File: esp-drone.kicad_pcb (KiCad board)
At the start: 4 copper layers, 72.8 x 72.8 mm, 0 parts

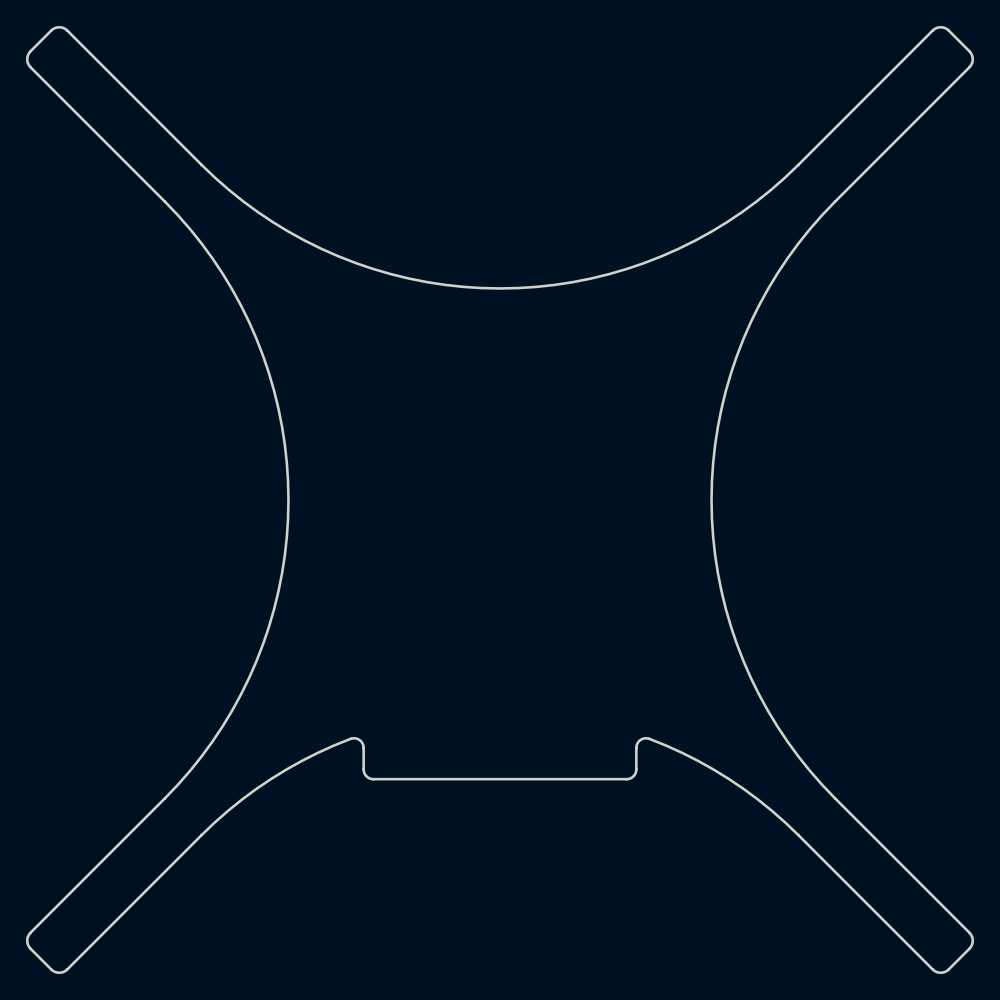
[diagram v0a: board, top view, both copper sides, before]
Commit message: .
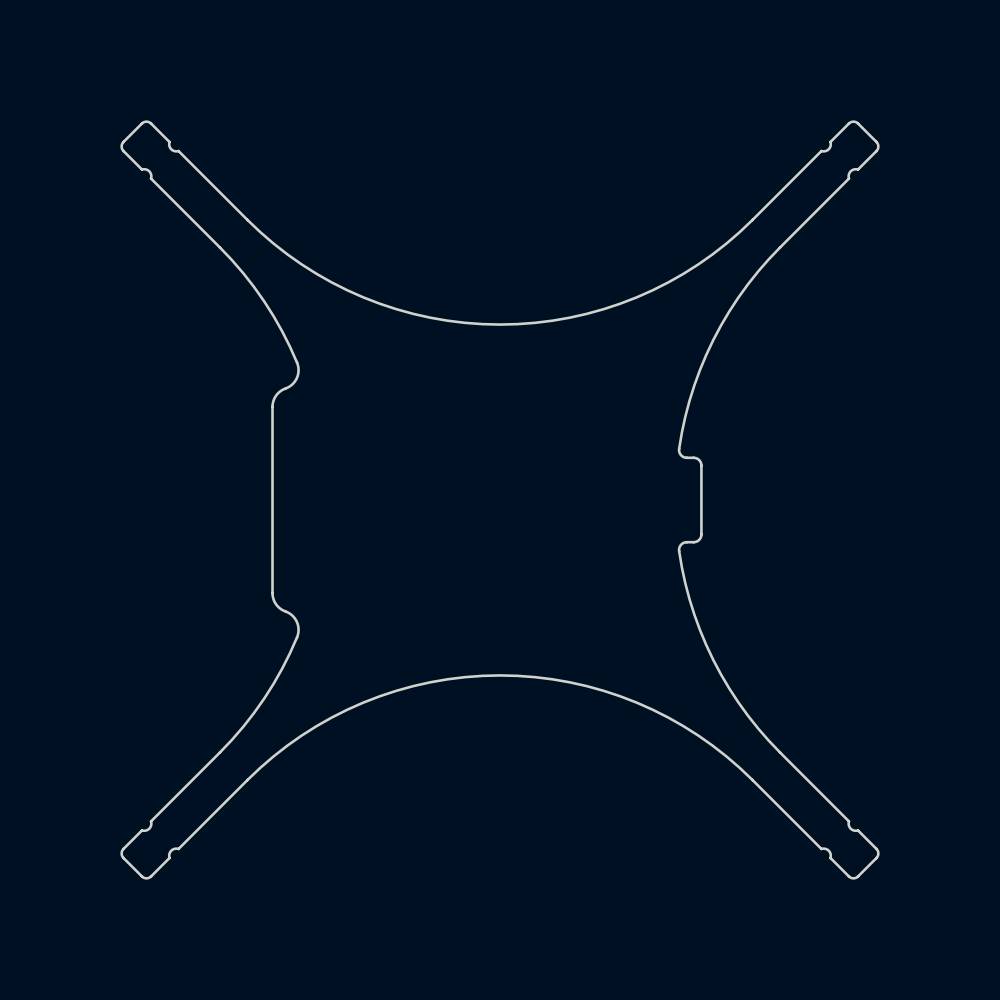
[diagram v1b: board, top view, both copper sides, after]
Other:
- board size 72.8 x 72.8 mm -> 58.3 x 58.3 mm
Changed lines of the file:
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@@
   (general
     (thickness 1.6)
-    (drawings 32)
+    (drawings 54)
     (tracks 0)
     (zones 0)
@@
     (uvia_drill 0.1)
   )
-  (gr_arc (start 0 48.790367) (end 22.98097 25.809397) (angle -24.24756936) (layer Edge.Cuts) (width 0.2))
-  (gr_line (start -36.150834 33.322407) (end -25.809397 22.98097) (layer Edge.Cuts) (width 0.2))
-  (gr_line (start -33.322407 36.150834) (end -22.98097 25.809397) (layer Edge.Cuts) (width 0.2))
-  (gr_line (start 22.98097 25.809397) (end 33.322407 36.150834) (layer Edge.Cuts) (width 0.2))
-  (gr_line (start -33.322407 -36.150834) (end -22.98097 -25.809397) (layer Edge.Cuts) (width 0.2))
-  (gr_line (start 22.98097 -25.809397) (end 33.322407 -36.150834) (layer Edge.Cuts) (width 0.2))
-  (gr_line (start 25.809397 22.98097) (end 36.150834 33.322407) (layer Edge.Cuts) (width 0.2))
-  (gr_arc (start 0 48.790367) (end -11.515748 18.398962) (angle -24.24756936) (layer Edge.Cuts) (width 0.2))
-  (gr_line (start -36.150834 -33.322407) (end -25.809397 -22.98097) (layer Edge.Cuts) (width 0.2))
-  (gr_line (start 25.809397 -22.98097) (end 36.150834 -33.322407) (layer Edge.Cuts) (width 0.2))
-  (gr_arc (start 35.532115 33.941125) (end 36.150834 34.559843) (angle -90) (layer Edge.Cuts) (width 0.2))
-  (gr_arc (start -9.75 20.749999) (end -10.5 20.749999) (angle -90) (layer Edge.Cuts) (width 0.2))
-  (gr_arc (start -11.249999 19.100302) (end -10.499999 19.100302) (angle -110.7524306) (layer Edge.Cuts) (width 0.2))
-  (gr_arc (start -48.790367 0) (end -25.809397 22.98097) (angle -90) (layer Edge.Cuts) (width 0.2))
-  (gr_arc (start 35.532115 -33.941125) (end 36.150834 -33.322407) (angle -90) (layer Edge.Cuts) (width 0.2))
-  (gr_arc (start -35.532115 -33.941125) (end -36.150834 -34.559843) (angle -90) (layer Edge.Cuts) (width 0.2))
-  (gr_arc (start -33.941125 -35.532115) (end -33.322407 -36.150834) (angle -90) (layer Edge.Cuts) (width 0.2))
-  (gr_arc (start -35.532115 33.941125) (end -36.150834 33.322407) (angle -90) (layer Edge.Cuts) (width 0.2))
-  (gr_arc (start -33.941125 35.532115) (end -34.559843 36.150834) (angle -90) (layer Edge.Cuts) (width 0.2))
-  (gr_arc (start 9.75 20.75) (end 9.75 21.5) (angle -90) (layer Edge.Cuts) (width 0.2))
-  (gr_line (start 10.5 20.75) (end 10.5 19.100302) (layer Edge.Cuts) (width 0.2))
-  (gr_line (start 34.559843 -36.150834) (end 36.150834 -34.559843) (layer Edge.Cuts) (width 0.2))
-  (gr_line (start -10.5 20.749999) (end -10.5 19.100302) (layer Edge.Cuts) (width 0.2))
-  (gr_line (start -36.150834 -34.559843) (end -34.559843 -36.150834) (layer Edge.Cuts) (width 0.2))
-  (gr_line (start -9.75 21.499999) (end 9.75 21.5) (layer Edge.Cuts) (width 0.2))
-  (gr_line (start 36.150834 34.559843) (end 34.559843 36.150834) (layer Edge.Cuts) (width 0.2))
-  (gr_arc (start 0 -48.790367) (end -22.98097 -25.809397) (angle -90) (layer Edge.Cuts) (width 0.2))
-  (gr_arc (start 11.25 19.100302) (end 11.515748 18.398962) (angle -110.7524306) (layer Edge.Cuts) (width 0.2))
-  (gr_line (start -34.559843 36.150834) (end -36.150834 34.559843) (layer Edge.Cuts) (width 0.2))
-  (gr_arc (start 48.790367 0) (end 25.809397 -22.98097) (angle -90) (layer Edge.Cuts) (width 0.2))
-  (gr_arc (start 33.941125 35.532115) (end 33.322407 36.150834) (angle -90) (layer Edge.Cuts) (width 0.2))
-  (gr_arc (start 33.941125 -35.532115) (end 34.559843 -36.150834) (angle -90) (layer Edge.Cuts) (width 0.2))
+  (gr_arc (start 24.926386 -27.399594) (end 24.756735 -26.876413) (angle -125.9286164) (layer Edge.Cuts) (width 0.2))
+  (gr_arc (start 41.013498 0) (end 13.796612 3.935873) (angle -36.77324075) (layer Edge.Cuts) (width 0.2))
+  (gr_line (start -24.756735 26.876413) (end -19.444817 21.564832) (layer Edge.Cuts) (width 0.2))
+  (gr_arc (start 41.013498 0) (end 21.56868 -19.446055) (angle -36.77324075) (layer Edge.Cuts) (width 0.2))
+  (gr_arc (start -24.926386 27.399594) (end -24.756735 26.876413) (angle -125.9286164) (layer Edge.Cuts) (width 0.2))
+  (gr_line (start -28.992233 26.869135) (end -27.570831 25.447823) (layer Edge.Cuts) (width 0.2))
+  (gr_line (start -26.877988 24.755025) (end -21.56868 19.446055) (layer Edge.Cuts) (width 0.2))
+  (gr_line (start 25.449578 -27.569211) (end 26.87098 -28.990522) (layer Edge.Cuts) (width 0.2))
+  (gr_arc (start -41.013498 0) (end -21.56868 19.446055) (angle -22.3819565) (layer Edge.Cuts) (width 0.2))
+  (gr_line (start 19.444817 -21.564832) (end 24.756735 -26.876413) (layer Edge.Cuts) (width 0.2))
+  (gr_line (start -26.87098 28.990522) (end -25.449578 27.569211) (layer Edge.Cuts) (width 0.2))
+  (gr_line (start 15.513498 2.649999) (end 15.513498 -2.65) (layer Edge.Cuts) (width 0.2))
+  (gr_arc (start -16.021337 -7.168813) (end -16.517418 -8.584406) (angle -70.68749723) (layer Edge.Cuts) (width 0.2))
+  (gr_arc (start 14.913498 2.649999) (end 14.913498 3.249999) (angle -90) (layer Edge.Cuts) (width 0.2))
+  (gr_arc (start 0 -41.010888) (end -19.444817 -21.564832) (angle -89.99635326) (layer Edge.Cuts) (width 0.2))
+  (gr_arc (start -41.013498 0) (end -15.628883 -10.576923) (angle -22.38195842) (layer Edge.Cuts) (width 0.2))
+  (gr_line (start 19.444817 21.564832) (end 24.756735 26.876413) (layer Edge.Cuts) (width 0.2))
+  (gr_arc (start -27.40118 24.924642) (end -27.570831 25.447823) (angle -125.9286164) (layer Edge.Cuts) (width 0.2))
+  (gr_arc (start -17.013498 10) (end -15.628883 10.576923) (angle -93.30732713) (layer Edge.Cuts) (width 0.2))
+  (gr_line (start 21.56868 19.446055) (end 26.877988 24.755025) (layer Edge.Cuts) (width 0.2))
+  (gr_line (start 21.56868 -19.446055) (end 26.877988 -24.755025) (layer Edge.Cuts) (width 0.2))
+  (gr_line (start -28.992233 -26.869135) (end -27.570831 -25.447823) (layer Edge.Cuts) (width 0.2))
+  (gr_arc (start -17.013498 -10) (end -16.517418 -8.584406) (angle -93.30736218) (layer Edge.Cuts) (width 0.2))
+  (gr_line (start -17.521337 -7.168813) (end -17.521337 7.168814) (layer Edge.Cuts) (width 0.2))
+  (gr_line (start -24.756735 -26.876413) (end -19.444817 -21.564832) (layer Edge.Cuts) (width 0.2))
+  (gr_line (start 27.570831 -25.447823) (end 28.992233 -26.869135) (layer Edge.Cuts) (width 0.2))
+  (gr_line (start 14.913498 -3.25) (end 14.390435 -3.25) (layer Edge.Cuts) (width 0.2))
+  (gr_arc (start -16.021337 7.168813) (end -17.521337 7.168814) (angle -70.68751853) (layer Edge.Cuts) (width 0.2))
+  (gr_arc (start 27.40118 -24.924642) (end 27.570831 -25.447823) (angle -125.9286164) (layer Edge.Cuts) (width 0.2))
+  (gr_line (start 27.570831 25.447823) (end 28.992233 26.869135) (layer Edge.Cuts) (width 0.2))
+  (gr_arc (start 14.390435 -3.85) (end 13.796612 -3.935873) (angle -98.22858262) (layer Edge.Cuts) (width 0.2))
+  (gr_arc (start 14.913498 -2.65) (end 15.513498 -2.65) (angle -90) (layer Edge.Cuts) (width 0.2))
+  (gr_arc (start 14.390435 3.849999) (end 14.390435 3.249999) (angle -98.22858262) (layer Edge.Cuts) (width 0.2))
+  (gr_line (start -26.877988 -24.755025) (end -21.56868 -19.446055) (layer Edge.Cuts) (width 0.2))
+  (gr_arc (start -24.926386 -27.399594) (end -25.449578 -27.569211) (angle -125.9286164) (layer Edge.Cuts) (width 0.2))
+  (gr_line (start 25.449578 27.569211) (end 26.87098 28.990522) (layer Edge.Cuts) (width 0.2))
+  (gr_arc (start 27.40118 24.924642) (end 26.877988 24.755025) (angle -125.9286164) (layer Edge.Cuts) (width 0.2))
+  (gr_line (start 14.390435 3.249999) (end 14.913498 3.249999) (layer Edge.Cuts) (width 0.2))
+  (gr_line (start -26.87098 -28.990522) (end -25.449578 -27.569211) (layer Edge.Cuts) (width 0.2))
+  (gr_arc (start -27.40118 -24.924642) (end -26.877988 -24.755025) (angle -125.9286164) (layer Edge.Cuts) (width 0.2))
+  (gr_arc (start 24.926386 27.399594) (end 25.449578 27.569211) (angle -125.9286164) (layer Edge.Cuts) (width 0.2))
+  (gr_arc (start 0 41.010888) (end 19.444817 21.564832) (angle -89.99635326) (layer Edge.Cuts) (width 0.2))
+  (gr_arc (start -27.224522 -28.636958) (end -26.87098 -28.990522) (angle -90) (layer Edge.Cuts) (width 0.2))
+  (gr_arc (start -28.63869 -27.222699) (end -28.992255 -27.576241) (angle -90) (layer Edge.Cuts) (width 0.2))
+  (gr_arc (start 28.63869 -27.222699) (end 28.992233 -26.869135) (angle -90) (layer Edge.Cuts) (width 0.2))
+  (gr_arc (start 28.63869 27.222699) (end 28.992255 27.576241) (angle -90) (layer Edge.Cuts) (width 0.2))
+  (gr_line (start 28.992255 27.576241) (end 27.578087 28.9905) (layer Edge.Cuts) (width 0.2))
+  (gr_arc (start 27.224522 -28.636958) (end 27.578087 -28.9905) (angle -90) (layer Edge.Cuts) (width 0.2))
+  (gr_arc (start 27.224522 28.636958) (end 26.87098 28.990522) (angle -90) (layer Edge.Cuts) (width 0.2))
+  (gr_arc (start -27.224522 28.636958) (end -27.578087 28.9905) (angle -90) (layer Edge.Cuts) (width 0.2))
+  (gr_line (start 27.578087 -28.9905) (end 28.992255 -27.576241) (layer Edge.Cuts) (width 0.2))
+  (gr_arc (start -28.63869 27.222699) (end -28.992233 26.869135) (angle -90) (layer Edge.Cuts) (width 0.2))
+  (gr_line (start -27.578087 -28.9905) (end -28.992255 -27.576241) (layer Edge.Cuts) (width 0.2))
+  (gr_line (start -28.992255 27.576241) (end -27.578087 28.9905) (layer Edge.Cuts) (width 0.2))
 )
